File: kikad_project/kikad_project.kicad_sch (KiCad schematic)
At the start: 50 parts, among them IC1 HCPL-2531, IC2 HCPL-2531, IC3 HCPL-2531, J1 236-102, J10 236-104, J11 236-104, J12 236-744, J13 236-102, J14 236-102, J15 236-102, J16 236-102, J17 236-744, J18 236-102, J2 236-104, J3 236-102, J4 236-102, J5 236-744, J6 236-102, J7 236-102, J8 236-744, J9 236-102, Q2 IRF5305PbF, U1 NRF24L01_Breakout, U12 CD40109BE, U2 STM32F103C8T6, U3 L7805, U4 L7805, X1 3522-2

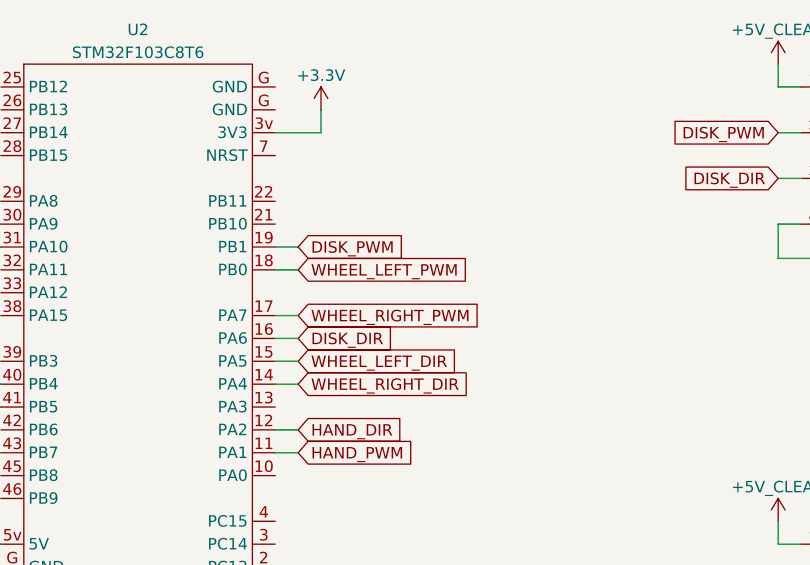
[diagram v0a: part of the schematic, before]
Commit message: PCB ready
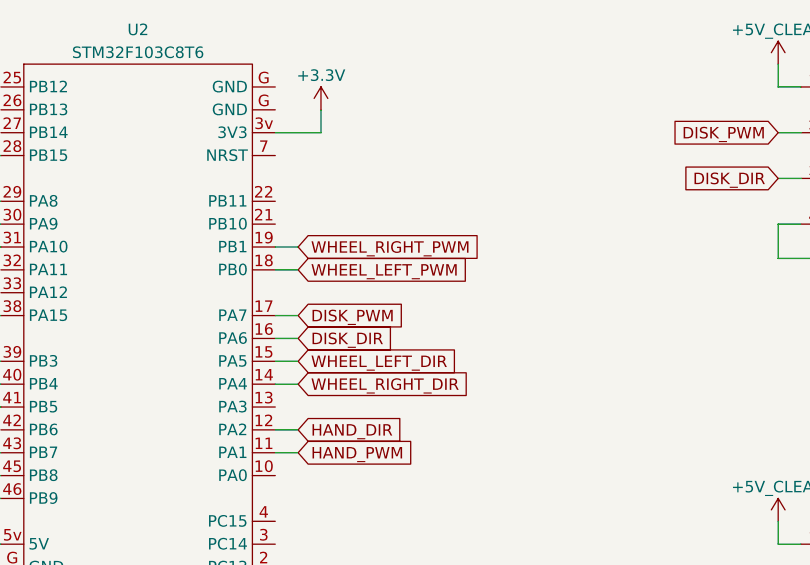
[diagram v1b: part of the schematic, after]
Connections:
- net DISK_PWM: now also U2.17 (PA7); no longer U2.19 (PB1)
- net WHEEL_RIGHT_PWM: now also U2.19 (PB1); no longer U2.17 (PA7)
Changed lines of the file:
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@@
+    )
+  )
+  (global_label "WHEEL_RIGHT_PWM" (shape input) (at 144.78 40.64 0) (fields_autoplaced)
+    (effects (font (size 1.27 1.27)) (justify left))
+    (property "Intersheetrefs" "${INTERSHEET_REFS}" (at 165.4241 40.64 0)
+      (effects (font (size 1.27 1.27)) (justify left) hide)
     )
   )
@@
     (property "Intersheetrefs" "${INTERSHEET_REFS}" (at 102.6667 38.1 0)
       (effects (font (size 1.27 1.27)) (justify right) hide)
+    )
+  )
+  (global_label "DISK_PWM" (shape input) (at 144.78 48.26 0) (fields_autoplaced)
+    (effects (font (size 1.27 1.27)) (justify left))
+    (property "Intersheetrefs" "${INTERSHEET_REFS}" (at 157.2599 48.26 0)
+      (effects (font (size 1.27 1.27)) (justify left) hide)
     )
   )
@@
     (effects (font (size 1.27 1.27)) (justify left))
     (property "Intersheetrefs" "${INTERSHEET_REFS}" (at 163.1865 53.34 0)
-      (effects (font (size 1.27 1.27)) (justify left) hide)
-    )
-  )
-  (global_label "WHEEL_RIGHT_PWM" (shape input) (at 144.78 48.26 0) (fields_autoplaced)
-    (effects (font (size 1.27 1.27)) (justify left))
-    (property "Intersheetrefs" "${INTERSHEET_REFS}" (at 165.4241 48.26 0)
       (effects (font (size 1.27 1.27)) (justify left) hide)
     )
@@
       (effects (font (size 1.27 1.27)) (justify left) hide)
     )
-  )
-  (global_label "DISK_PWM" (shape input) (at 144.78 40.64 0) (fields_autoplaced)
-    (effects (font (size 1.27 1.27)) (justify left))
-    (property "Intersheetrefs" "${INTERSHEET_REFS}" (at 157.2599 40.64 0)
-      (effects (font (size 1.27 1.27)) (justify left) hide)
-    )
